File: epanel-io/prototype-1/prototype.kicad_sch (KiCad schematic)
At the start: 20 parts, among them J1 Screw_Terminal_01x04, J2 Conn_01x02_Male, J3 Screw_Terminal_01x02, J4 Conn_01x03_Male, Q1 IRF830, U1 4N35, U2 H11AA1

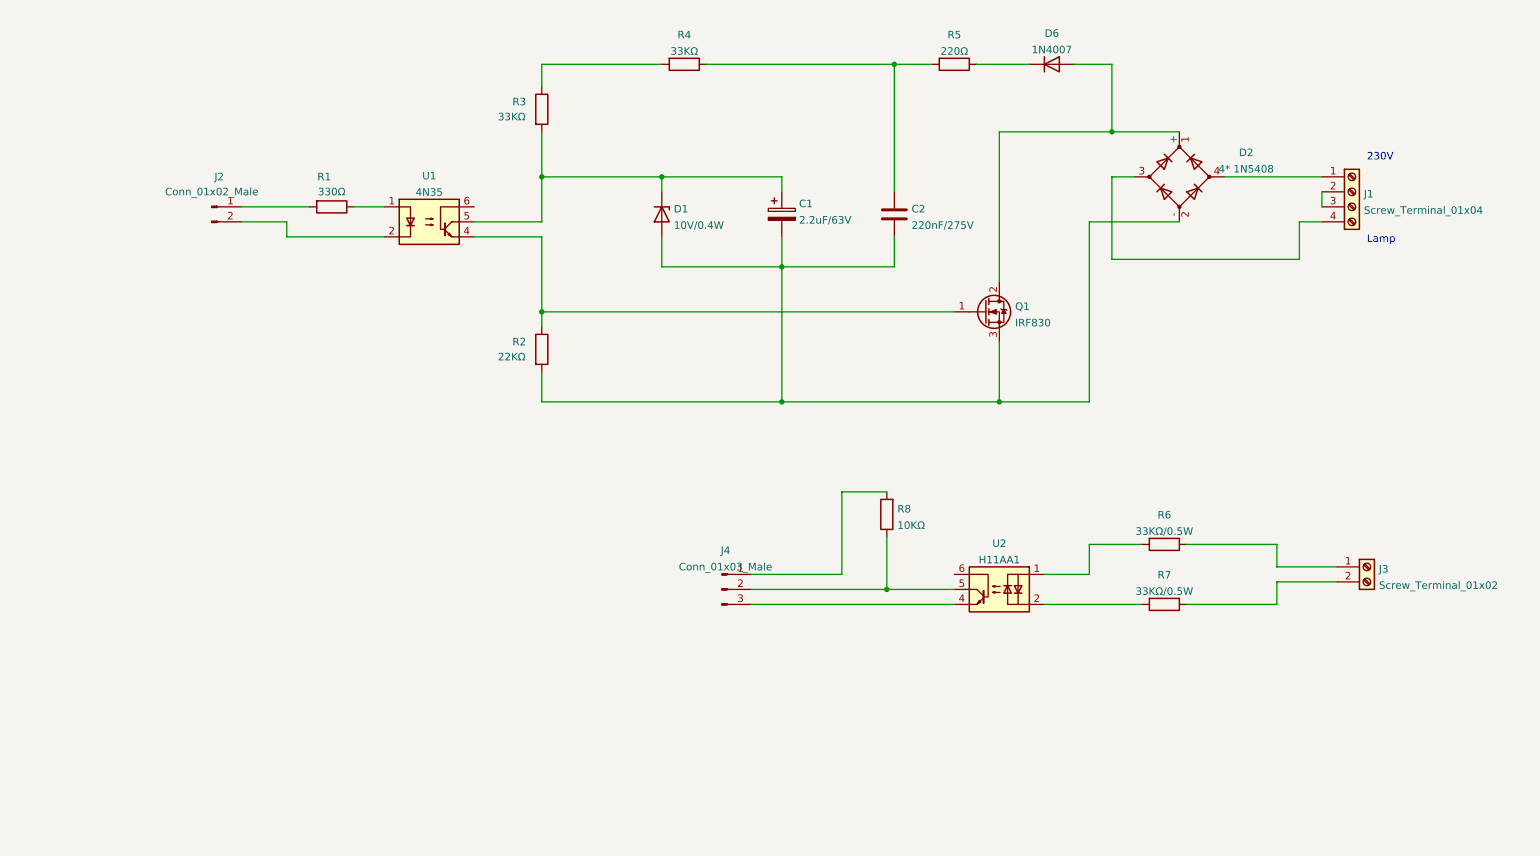
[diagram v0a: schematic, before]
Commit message: schematic wip
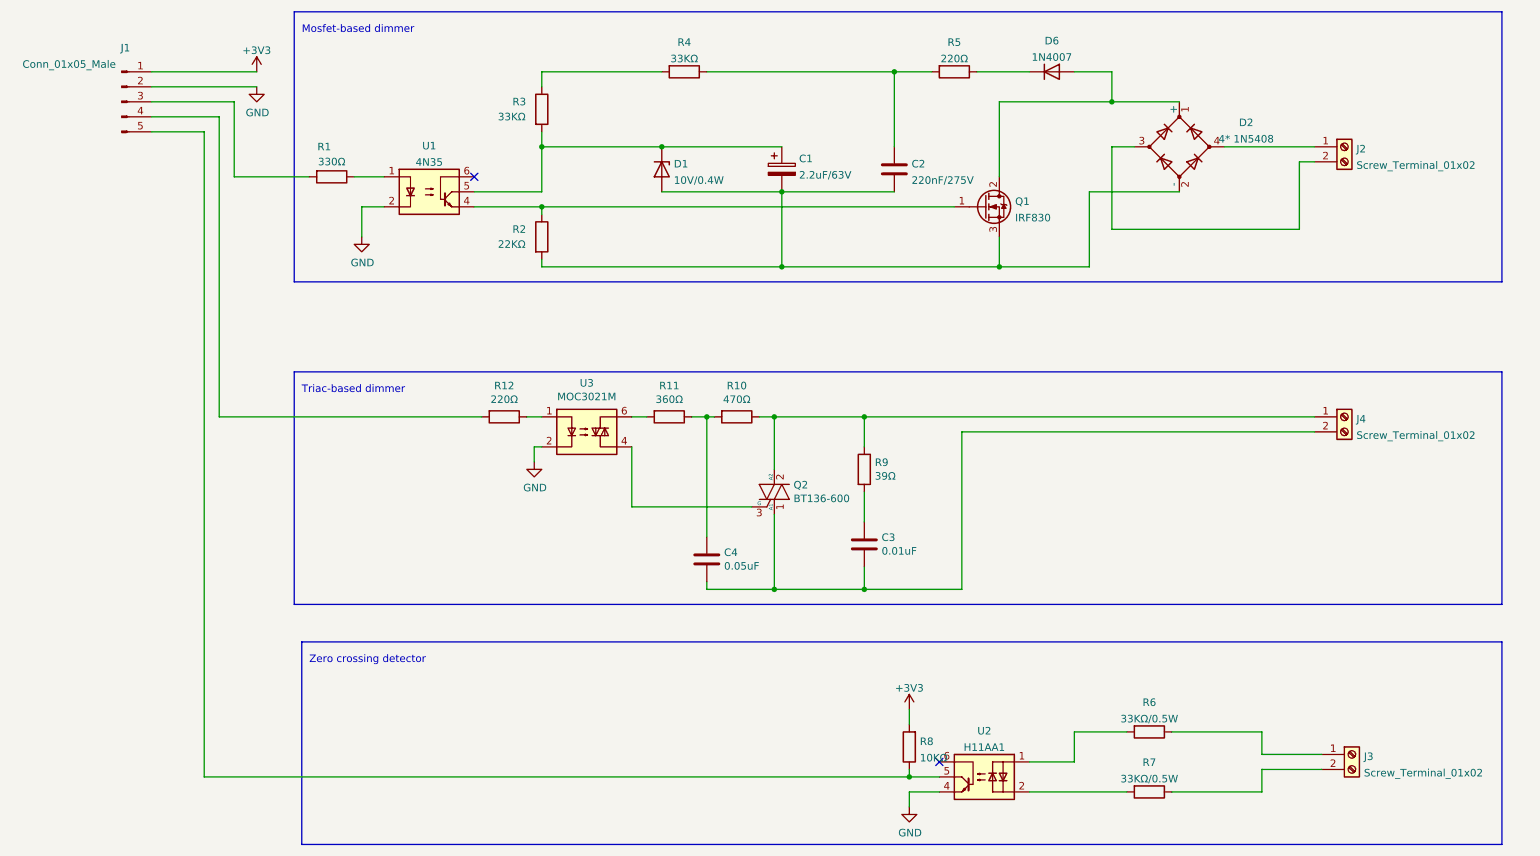
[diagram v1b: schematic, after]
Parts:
- removed J1: Screw_Terminal_01x04, symbol Connector:Screw_Terminal_01x04
- removed J2: Conn_01x02_Male, symbol Connector:Conn_01x02_Male
- removed J4: Conn_01x03_Male, symbol Connector:Conn_01x03_Male
- added C3: 0.01uF, Capacitor_THT:C_Rect_L9.0mm_W2.5mm_P7.50mm_MKT, symbol Device:C
- added C4: 0.05uF, Capacitor_SMD:C_2220_5650Metric_Pad1.97x5.40mm_HandSolder, symbol Device:C
- added J1: Conn_01x05_Male, symbol Connector:Conn_01x05_Male
- added J2, J4: Screw_Terminal_01x02, symbol Connector:Screw_Terminal_01x02
- added Q2: BT136-600, Package_TO_SOT_THT:TO-220-3_Vertical, symbol Triac_Thyristor:BT136-600
- added R10: 470Ω, Resistor_SMD:R_1206_3216Metric_Pad1.42x1.75mm_HandSolder, symbol Device:R
- added R11: 360Ω, Resistor_SMD:R_1206_3216Metric_Pad1.42x1.75mm_HandSolder, symbol Device:R
- added R12: 220Ω, Resistor_SMD:R_1206_3216Metric_Pad1.42x1.75mm_HandSolder, symbol Device:R
- added R9: 39Ω, Resistor_THT:R_Axial_DIN0204_L3.6mm_D1.6mm_P7.62mm_Horizontal, symbol Device:R
- added U3: MOC3021M, Package_DIP:DIP-6_W8.89mm_SMDSocket_LongPads, symbol Relay_SolidState:MOC3021M
- R1, R2, R3, R4, R5, R8: footprint (none) -> Resistor_SMD:R_1206_3216Metric_Pad1.42x1.75mm_HandSolder
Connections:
- net +3V3: now reaches R8.2
- net +3V3: now also J1.1 (Pin_1)
- net at R8.1, U2.5: now also J1.5 (Pin_5)
- net GND: now reaches U2.4
- net GND: now also U1.2, J1.2 (Pin_2), U3.2
- net at D2.4: now also J2.1 (Pin_1)
- net at D2.3: now also J2.2 (Pin_2)
- net at R1.2: now also J1.3 (Pin_3)
- new net: C4.1, R10.2, R11.1
- new net: C3.2, C4.2, J4.2 (Pin_2), Q2.1 (A1)
- new net: R11.2, U3.6
- new net: J4.1 (Pin_1), Q2.2 (A2), R10.1, R9.1
- new net: C3.1, R9.2
- new net: R12.1, U3.1
- new net: Q2.3 (G), U3.4
- new net: J1.4 (Pin_4), R12.2
- no-connect marks 0 -> 2
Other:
- note added: "Mosfet-based dimmer"
- note added: "Triac-based dimmer"
- note added: "Zero crossing detector"
- note removed: "230V"
- note removed: "Lamp"
- moved on the sheet: C1, C2, D1, D2, D6, J3, Q1, R1, R2, R4, R5, R6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

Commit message: add JLPCB refs + footprints
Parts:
- J1: footprint (none) -> Connector_PinHeader_2.54mm:PinHeader_1x05_P2.54mm_Vertical
- J2, J3, J4: footprint (none) -> TerminalBlock:TerminalBlock_bornier-2_P5.08mm
- R1: footprint Resistor_SMD:R_1206_3216Metric_Pad1.42x1.75mm_HandSolder -> Resistor_SMD:R_0603_1608Metric; JLCPCB (none) -> C23138
- R10: footprint Resistor_SMD:R_1206_3216Metric_Pad1.42x1.75mm_HandSolder -> Resistor_SMD:R_0603_1608Metric; JLCPCB (none) -> C23179
- R11: footprint Resistor_SMD:R_1206_3216Metric_Pad1.42x1.75mm_HandSolder -> Resistor_SMD:R_0603_1608Metric; JLCPCB (none) -> C25194
- R12, R5: footprint Resistor_SMD:R_1206_3216Metric_Pad1.42x1.75mm_HandSolder -> Resistor_SMD:R_0603_1608Metric; JLCPCB (none) -> C22962
- R2: footprint Resistor_SMD:R_1206_3216Metric_Pad1.42x1.75mm_HandSolder -> Resistor_SMD:R_0603_1608Metric; JLCPCB (none) -> C31850
- R3, R4: footprint Resistor_SMD:R_1206_3216Metric_Pad1.42x1.75mm_HandSolder -> Resistor_SMD:R_0603_1608Metric; JLCPCB (none) -> C4216
- R6, R7: footprint (none) -> Resistor_SMD:R_0805_2012Metric; JLCPCB (none) -> C966118
- R8: footprint Resistor_SMD:R_1206_3216Metric_Pad1.42x1.75mm_HandSolder -> Resistor_SMD:R_0603_1608Metric; JLCPCB (none) -> C25804
- R9: footprint Resistor_THT:R_Axial_DIN0204_L3.6mm_D1.6mm_P7.62mm_Horizontal -> Resistor_SMD:R_0603_1608Metric; JLCPCB (none) -> C23154
- U1: footprint Package_DIP:DIP-6_W7.62mm -> (none); JLCPCB (none) -> C115444
- U2: footprint Package_DIP:DIP-6_W7.62mm -> (none); JLCPCB (none) -> C184383
- U3: footprint Package_DIP:DIP-6_W8.89mm_SMDSocket_LongPads -> (none); JLCPCB (none) -> C115465
